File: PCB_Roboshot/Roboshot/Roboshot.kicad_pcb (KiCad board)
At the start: 2 copper layers, 78.3 x 91.9 mm, 30 parts, among them J2 Conn_01x08, J4 Conn_01x03, J6 Conn_01x04, Q1_LIGHT1 BC546, Q1_PCA1 BC546, Q2_PUMP_DC1 BC546, U1 7840-0000PR, U2 H

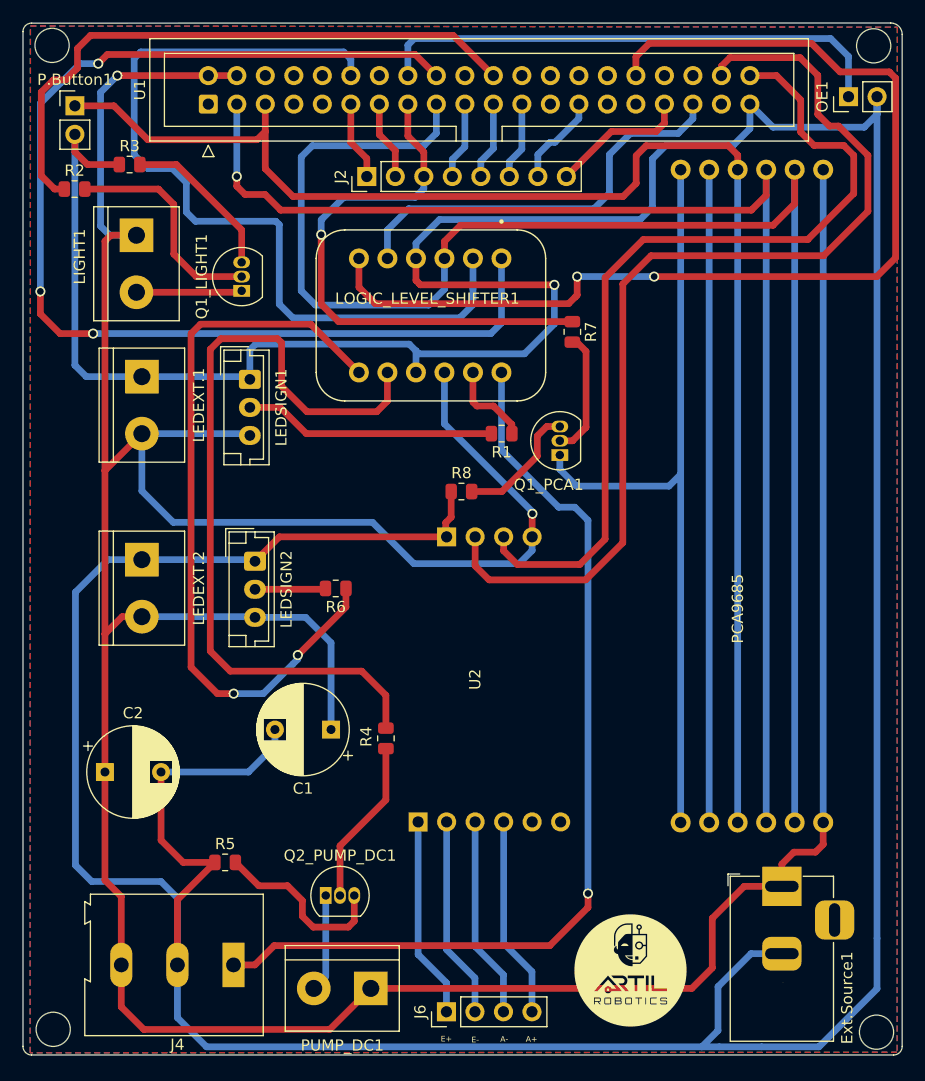
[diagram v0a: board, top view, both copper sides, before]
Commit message: Placa final_Roboshot
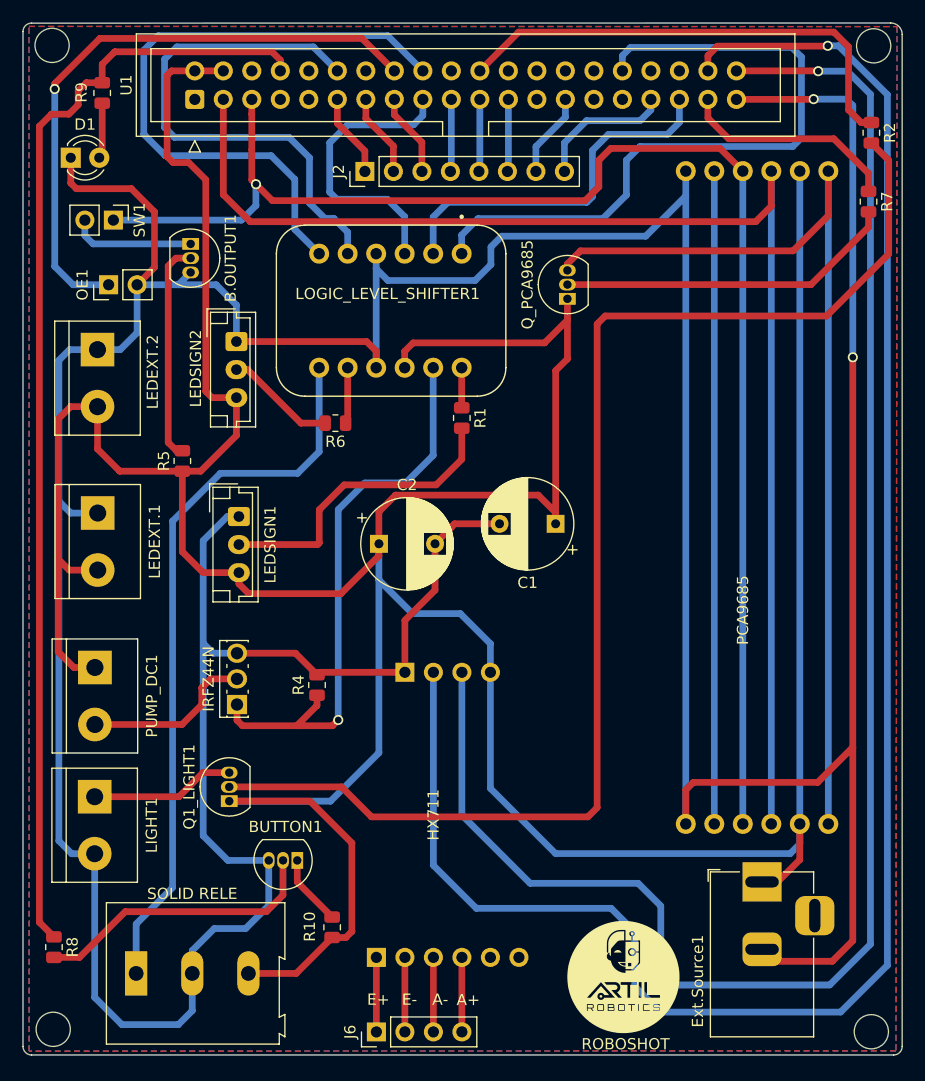
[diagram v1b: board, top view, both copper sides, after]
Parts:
- removed G: LOGO, Sensor:Sello1_artil
- removed J4: Conn_01x03, TerminalBlock:TerminalBlock_Altech_AK300-3_P5.00mm
- removed P.Button1: Conn_01x02, Connector_PinHeader_2.54mm:PinHeader_1x02_P2.54mm_Vertical
- removed Q1_PCA1, Q2_PUMP_DC1: BC546, Package_TO_SOT_THT:TO-92_Inline
- removed R3: R, Resistor_SMD:R_0805_2012Metric
- removed U2: H, DualChannel_HX711:Dual Channel
- added B.OUTPUT1: BC546, Package_TO_SOT_THT:TO-92_Inline, F.Cu at (239.2, 128.0)
- added BUTTON1: BC546, Package_TO_SOT_THT:TO-92_Inline, F.Cu at (248.7, 183.0)
- added D1: LED, LED_THT:LED_D3.0mm, F.Cu at (228.5, 120.3)
- added HX711: H, DualChannel_HX711:Dual Channel, F.Cu at (268.5, 191.6)
- added IRFZ44N: BSP89, Package_TO_SOT_THT:SIPAK_Vertical, F.Cu at (243.3, 169.1)
- added Q_PCA9685: BC546, Package_TO_SOT_THT:TO-92_Inline, F.Cu at (272.8, 132.9)
- added R10: R, Resistor_SMD:R_0805_2012Metric, F.Cu at (251.8, 188.9)
- added R9: R, Resistor_SMD:R_0805_2012Metric, F.Cu at (231.3, 114.6)
- added ROBOSHOT: ROBOSHOT, Symbol:Sello-ArtilRobotics, F.Cu at (277.8, 193.3)
- added SOLID RELE: Conn_01x03, TerminalBlock:TerminalBlock_Altech_AK300-3_P5.00mm, F.Cu at (234.4, 193.0)
- added SW1: SW_Push_Dual_x2, Connector_PinHeader_2.54mm:PinHeader_1x02_P2.54mm_Vertical, F.Cu at (232.3, 125.9)
- moved R2 71.2 mm to (299.9, 118.1), turned to -90 degrees
- moved OE1 68.0 mm to (231.9, 131.7)
- moved R8 54.5 mm to (227.0, 190.7), turned to -90 degrees
- moved LIGHT1 50.2 mm to (230.7, 177.3)
- moved Q1_LIGHT1 45.5 mm to (242.7, 177.7)
- moved PUMP_DC1 37.7 mm to (230.7, 165.8), turned to -90 degrees
- moved R5 36.0 mm to (238.5, 147.4), turned to 90 degrees
- moved C2 31.8 mm to (256.0, 154.7)
- moved R7 28.8 mm to (299.6, 124.3)
- moved C1 27.1 mm to (271.7, 153.0)
- moved LEDSIGN2 19.6 mm to (243.3, 136.7)
- moved LEDEXT.2 19.1 mm to (230.9, 137.4)
- moved R6 14.7 mm to (252.1, 144.0)
- moved LEDEXT.1 12.8 mm to (230.9, 152.0)
- moved LEDSIGN1 12.3 mm to (243.5, 152.3)
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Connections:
- LIGHT1 pad 1: +5V -> /LIGHT
- LIGHT1 pad 2: /LIGHT -> GND
- LOGIC_LEVEL_SHIFTER1 pad LV1: /GPIO24(GEN5) -> /GPIO12(PWM0)
- LOGIC_LEVEL_SHIFTER1 pad LV2: /GPIO18(GEN1)(PWM0) -> /GPIO19(SPI1_MISO)
- LOGIC_LEVEL_SHIFTER1 pad LV3: /GPIO19(SPI1_MISO) -> /GPIO18(GEN1)(PWM0)
- LOGIC_LEVEL_SHIFTER1 pad LV4: /GPIO12(PWM0) -> /GPIO24(GEN5)
- PCA9685 pad GND_1: /GND_PCA9685 -> GND
- PCA9685 pad GND_2: /GND_PCA9685 -> GND
- PCA9685 pad V+_1: +5V -> /2N_PCA9685
- PCA9685 pad V+_2: +5V -> /2N_PCA9685
- PCA9685 pad VCC_1: +3V3 -> +5V
- PCA9685 pad VCC_2: +3V3 -> +5V
- Q1_LIGHT1 pad 1: /LIGHT -> +5V
- Q1_LIGHT1 pad 3: Net-(Q1_LIGHT1-Pad3) -> /LIGHT
- R1 pad 1: /HV2 -> /HV1
- R4 pad 1: /HV3 -> /HV2
- R4 pad 2: Net-(Q2_PUMP_DC1-Pad2) -> GND
- R5 pad 1: GND -> +5V
- R6 pad 1: /HV4 -> /HV3
- R7 pad 1: /GPIO22(GEN3) -> /GPIO26
- R8 pad 1: GND -> /GPIO14(TXD0)
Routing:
- net +3V3: track 139.4 -> 26.0 mm
- net /GPIO14(TXD0): track 0.00 -> 99.9 mm
- net Net-(Q1_LIGHT1-Pad2): track 19.8 -> 116.4 mm
- net /2N_PCA9685: track 0.00 -> 87.7 mm
- net /HV1: track 85.4 -> 3.57 mm, vias 1 -> 0
- net /GPIO20(SPI1_MOSI): track 90.1 -> 164.7 mm, vias 0 -> 1
- net /GPIO21(SPI1_SCK): track 77.5 -> 149.0 mm, vias 0 -> 1
- net /GND_PCA9685: track 71.3 -> 0.00 mm
- net /HV3: track 71.2 -> 5.01 mm
- net /GPIO24(GEN5): track 104.6 -> 56.8 mm, vias 3 -> 0
- net /HV2: track 7.75 -> 51.3 mm, vias 0 -> 1
- net /GPIO22(GEN3): track 49.0 -> 7.44 mm, vias 1 -> 0
- net /GPIO12(PWM0): track 96.2 -> 62.5 mm, vias 2 -> 0
- net /GPIO18(GEN1)(PWM0): track 76.4 -> 47.3 mm
- net +5V: track 340.0 -> 368.1 mm, vias 2 -> 0
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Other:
- outline, holes or cut-outs redrawn

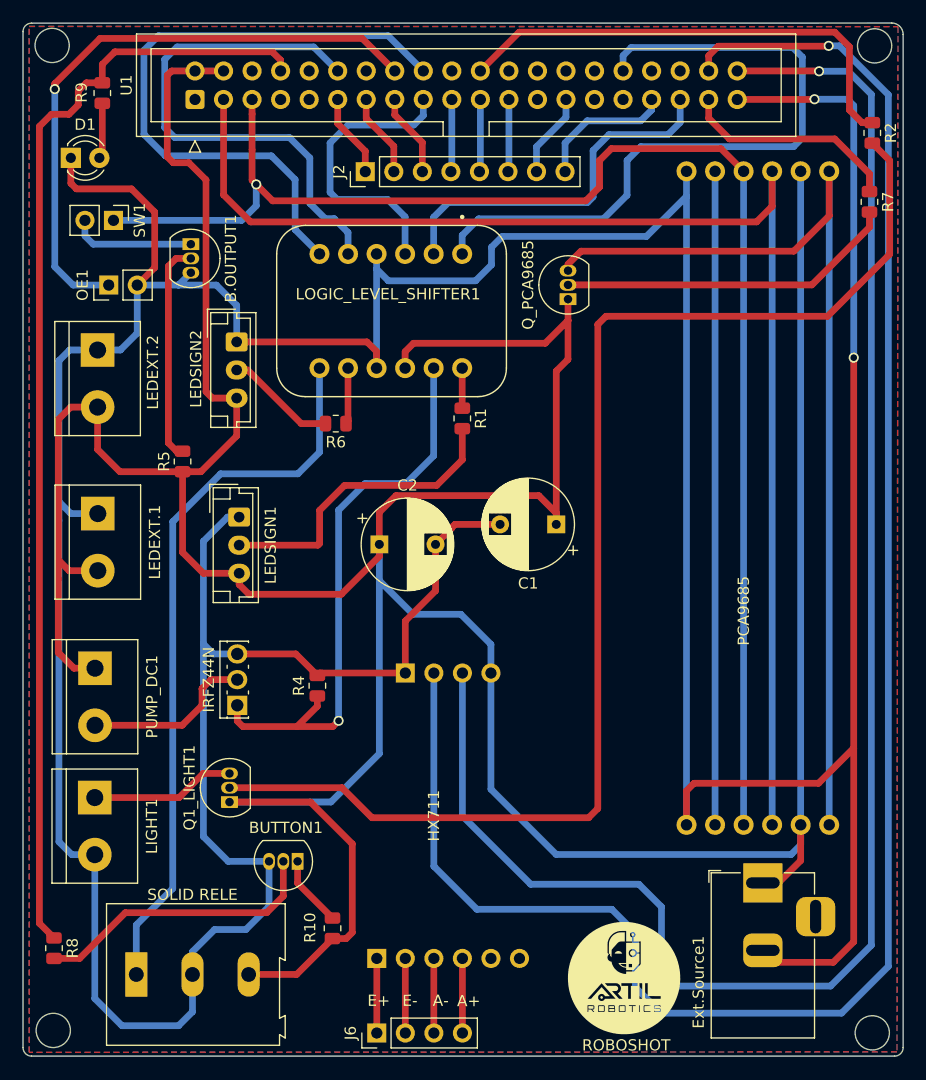
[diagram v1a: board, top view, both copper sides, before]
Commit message: Placa_reducida tamaño
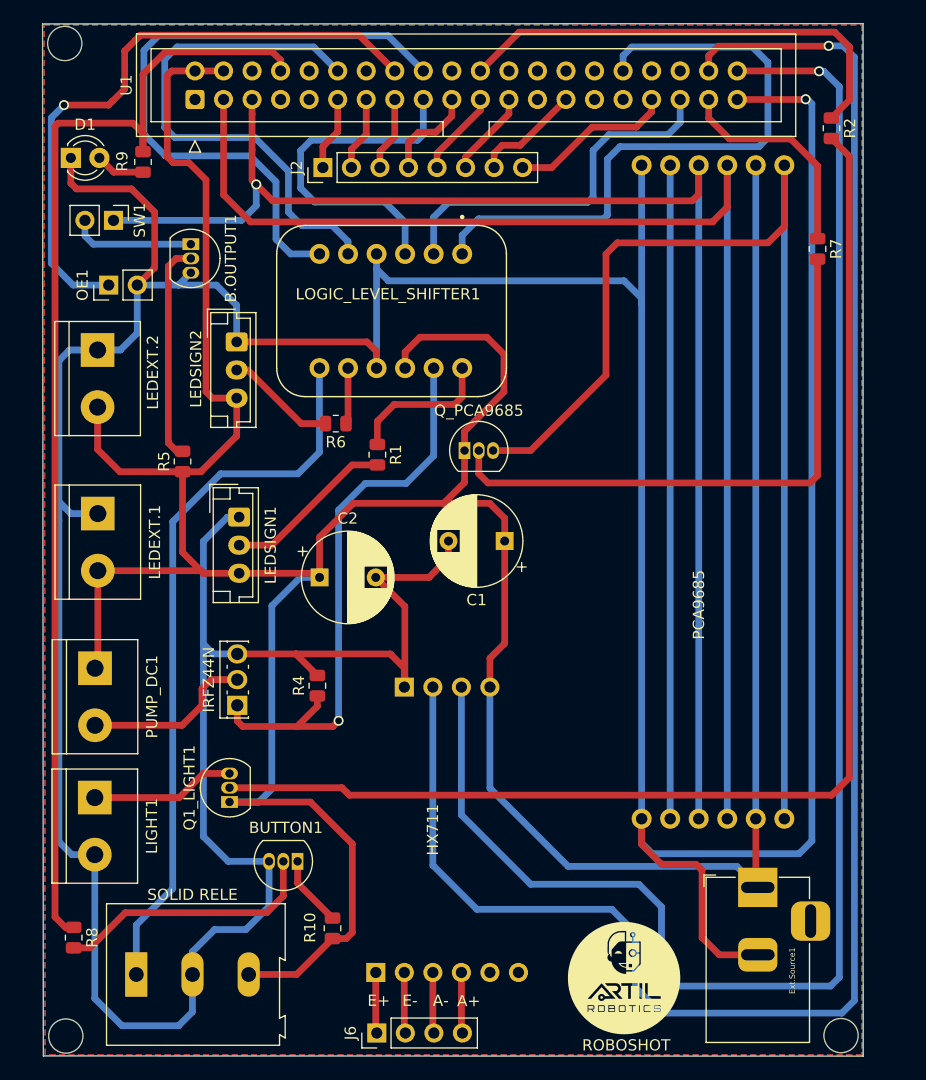
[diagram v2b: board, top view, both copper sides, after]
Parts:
- moved Q_PCA9685 16.3 mm to (263.6, 146.4), turned to 0 degrees
- moved R1 8.22 mm to (255.8, 146.8)
- moved R9 7.12 mm to (235.0, 120.7)
- moved R7 6.24 mm to (295.0, 128.4)
- moved C2 6.08 mm to (250.7, 157.7)
- moved C1 4.82 mm to (267.2, 154.4)
- moved PCA9685 4.03 mm to (284.9, 160.1)
- moved J2 3.79 mm to (251.0, 121.2)
- moved R2 3.65 mm to (296.2, 117.7)
- moved R8 1.99 mm to (228.8, 189.7)
- moved HX711 1.25 mm to (268.4, 192.8)
- moved Ext.Source1 0.60 mm to (289.7, 185.3)
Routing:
- net +5V: track 368.1 -> 320.9 mm
- net Net-(Q_PCA9685-Pad2): track 30.3 -> 52.1 mm
- net /2N_PCA9685: track 87.7 -> 104.1 mm
- net Net-(LEDSIGN1-Pad2): track 27.5 -> 15.3 mm
- net /HV1: track 3.57 -> 13.1 mm
- net GND: track 439.7 -> 433.5 mm, vias 2 -> 1
- net /GPIO3(SCL1): track 129.2 -> 123.8 mm
- net +3V3: track 26.0 -> 31.3 mm
- net /GPIO12(PWM0): track 62.5 -> 57.2 mm
- net /GPIO21(SPI1_SCK): track 149.0 -> 144.2 mm
- net /GPIO14(TXD0): track 99.9 -> 103.6 mm
- net /GPIO20(SPI1_MOSI): track 164.7 -> 161.2 mm
- net /GPIO2(SDA1): track 120.2 -> 116.8 mm
- net Net-(Q1_LIGHT1-Pad2): track 116.4 -> 113.6 mm
- net /GPIO13(PWM1): track 12.4 -> 14.6 mm
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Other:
- board size 78.3 x 91.9 mm -> 73 x 91.9 mm

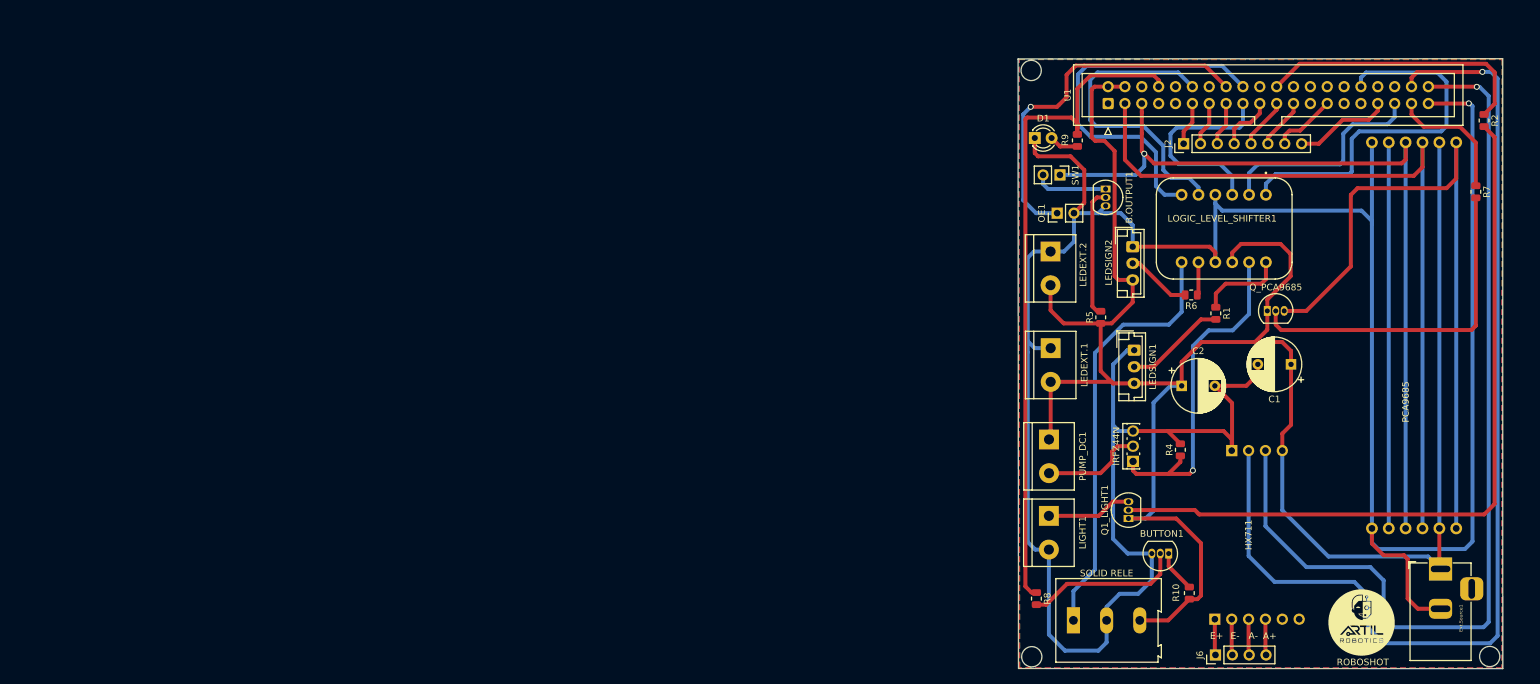
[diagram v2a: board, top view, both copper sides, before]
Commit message: revision de PCB
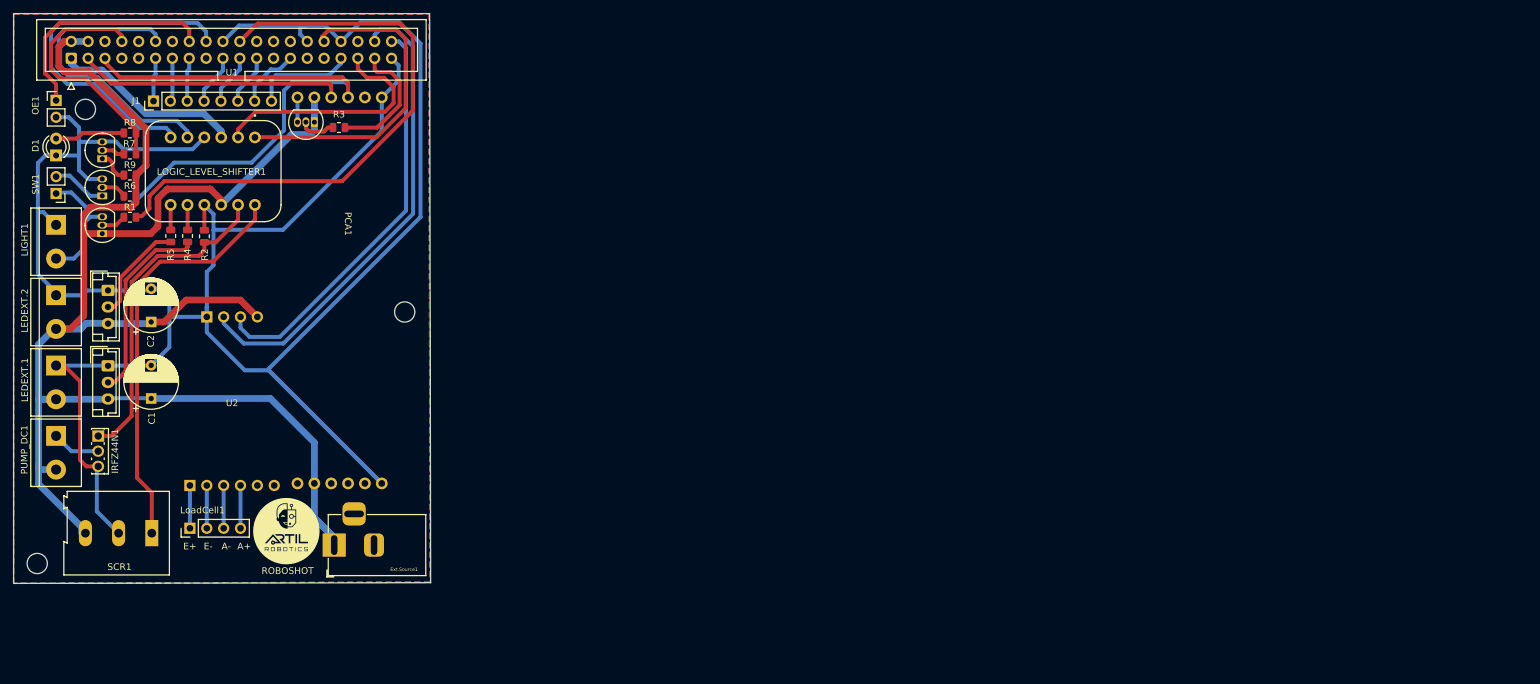
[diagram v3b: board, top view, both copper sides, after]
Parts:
- SCR1: renamed from SOLID RELE
- moved R1 204.6 mm to (92.2, 132.3), turned to 180 degrees
- moved C1 171.8 mm to (95.4, 159.6), turned to 90 degrees
- moved R9 171.6 mm to (92.2, 125.9), turned to 0 degrees
- moved R3 171.6 mm to (123.7, 118.8), turned to 180 degrees
- moved BUTTON1 171.3 mm to (88.0, 123.5), turned to 90 degrees
- moved Ext.Source1 166.7 mm to (123.0, 181.7), turned to 180 degrees
- moved LOGIC_LEVEL_SHIFTER1 166.3 mm to (104.7, 125.6)
- moved PCA1 162.6 mm to (124.6, 133.3), turned to -90 degrees
- moved ROBOSHOT 162.6 mm to (115.8, 179.6)
- moved Q1_LIGHT1 160.5 mm to (88.0, 134.7)
- moved U1 156.4 mm to (83.4, 108.3)
- moved IRFZ44N1 156.0 mm to (87.4, 165.2), turned to -90 degrees
- moved LIGHT1 155.9 mm to (81.1, 133.4)
- moved U2 155.7 mm to (113.9, 172.7)
- moved LoadCell1 155.7 mm to (101.2, 179.1)
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- renumbered IRFZ44N to IRFZ44N1, J2 to J1, J6 to LoadCell1, PCA9685 to PCA1, Q_PCA9685 to Q_PCA1, R2 to R1, R4 to R2, R7 to R3, R1 to R4, R6 to R5, R5 to R6, R8 to R7, R9 to R8, R10 to R9, HX711 to U2
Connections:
- LIGHT1 pad 1: /LIGHT -> GND
- LIGHT1 pad 2: GND -> /LIGHT
- LOGIC_LEVEL_SHIFTER1 pad HV1: /HV1 -> /HV4
- LOGIC_LEVEL_SHIFTER1 pad HV3: /HV3 -> /HV1
- LOGIC_LEVEL_SHIFTER1 pad HV4: /HV4 -> /HV3
- PUMP_DC1 pad 1: +5V -> /PUMP
- PUMP_DC1 pad 2: /PUMP -> +5V
- U1 pad 1: unconnected-(U1-Pad1) -> +3V3
- U1 pad 14: unconnected-(U1-Pad14) -> GND
- U1 pad 20: unconnected-(U1-Pad20) -> GND
- U1 pad 25: unconnected-(U1-Pad25) -> GND
- U1 pad 30: unconnected-(U1-Pad30) -> GND
- U1 pad 34: unconnected-(U1-Pad34) -> GND
- U1 pad 6: unconnected-(U1-Pad6) -> GND
- U1 pad 9: unconnected-(U1-Pad9) -> GND
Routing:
- net Net-(Q1_LIGHT1-Pad2): track 113.6 -> 3.75 mm
- net /2N_PCA9685: track 104.1 -> 3.86 mm
- net /GPIO20(SPI1_MOSI): track 161.2 -> 72.3 mm, vias 1 -> 0
- net /GPIO21(SPI1_SCK): track 144.2 -> 61.7 mm, vias 1 -> 0
- net /GPIO2(SDA1): track 116.8 -> 40.4 mm
- net /GPIO14(TXD0): track 103.6 -> 37.1 mm
- net +5V: track 320.9 -> 257.5 mm
- net GND: track 433.5 -> 373.5 mm, vias 1 -> 0
- net Net-(PCA1-PadOE_1): track 58.2 -> 0.00 mm
- net Net-(Q_PCA1-Pad2): track 52.1 -> 5.31 mm
- net /GPIO25(GEN6): track 41.8 -> 88.6 mm
- net /GPIO3(SCL1): track 123.8 -> 98.8 mm, vias 1 -> 0
- net /GPIO23(GEN4): track 55.8 -> 35.0 mm, vias 1 -> 0
- net Net-(BUTTON1-Pad2): track 23.7 -> 3.29 mm
- net Net-(B.OUTPUT1-Pad2): track 19.6 -> 3.45 mm
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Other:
- board size 73 x 91.9 mm -> 62.8 x 85.9 mm
